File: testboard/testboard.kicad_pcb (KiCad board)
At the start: 2 copper layers, 50.5 x 30 mm, 21 parts

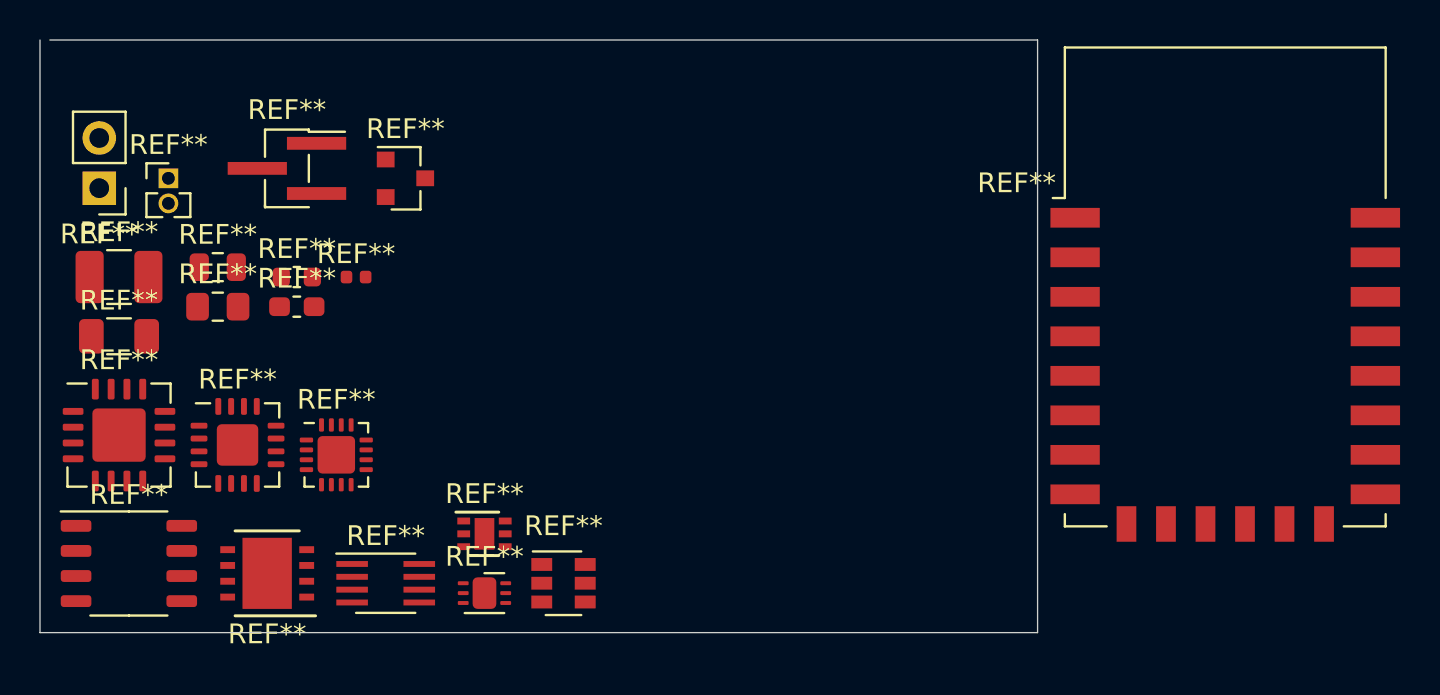
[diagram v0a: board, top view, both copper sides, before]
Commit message: testboard: First version
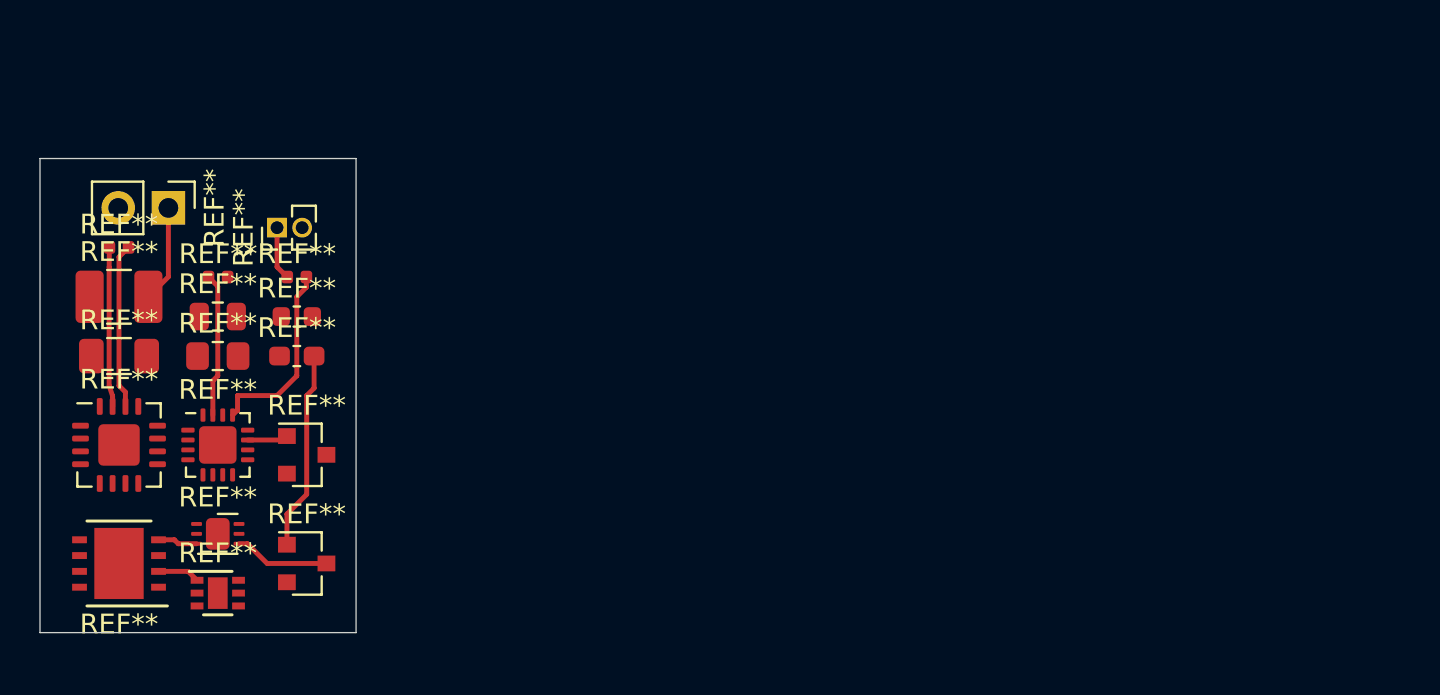
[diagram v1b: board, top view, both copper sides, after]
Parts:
- removed the REF** at (38.0, 49.0)
- removed the REF** at (60.5, 56.5)
- removed the REF** at (46.5, 35.5)
- removed the REF** at (94.0, 41.5)
- removed the REF** at (38.5, 55.5)
- removed the REF** at (51.5, 56.5)
- added REF**: SOT-23, Package_TO_SOT_SMD:SOT-23, F.Cu at (47.5, 55.5)
- added REF**: C_0402_1005Metric, Capacitor_SMD:C_0402_1005Metric, F.Cu at (38.0, 39.5)
- added REF**: C_0402_1005Metric, Capacitor_SMD:C_0402_1005Metric, F.Cu at (43.0, 41.0)
- moved REF** 14.9 mm to (47.5, 50.0)
- moved REF** 13.8 mm to (43.0, 57.0)
- moved REF** 13.8 mm to (43.0, 54.0)
- moved REF** 7.52 mm to (38.0, 55.5)
- moved REF** 6.04 mm to (46.0, 38.5), turned to 90 degrees
- moved REF** 6.02 mm to (43.0, 49.5)
- moved REF** 6.00 mm to (38.0, 49.5)
- moved REF** 3.64 mm to (40.5, 37.5), turned to 270 degrees
- moved REF** 3.00 mm to (47.0, 41.0)
- moved REF** 2.50 mm to (47.0, 45.0)
- moved REF** 2.50 mm to (43.0, 45.0)
- moved REF** 2.50 mm to (43.0, 43.0)
- moved REF** 2.00 mm to (47.0, 43.0)
- moved REF** 1.00 mm to (38.0, 42.0)
- moved REF** 1.00 mm to (38.0, 45.0)
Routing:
- net (no net): track 0.00 -> 62.3 mm
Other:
- board size 50.5 x 30 mm -> 16 x 24 mm
